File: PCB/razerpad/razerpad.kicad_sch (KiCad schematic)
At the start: 11 parts, among them SW1 SW_Push, SW2 SW_Push, SW3 SW_Push, SW4 RotaryEncoder_Switch, SW5 SW_Push, SW6 SW_Push, SW7 SW_Push, SW8 SW_Push, SW9 SW_Push, U1 XIAO-RP2040-DIP

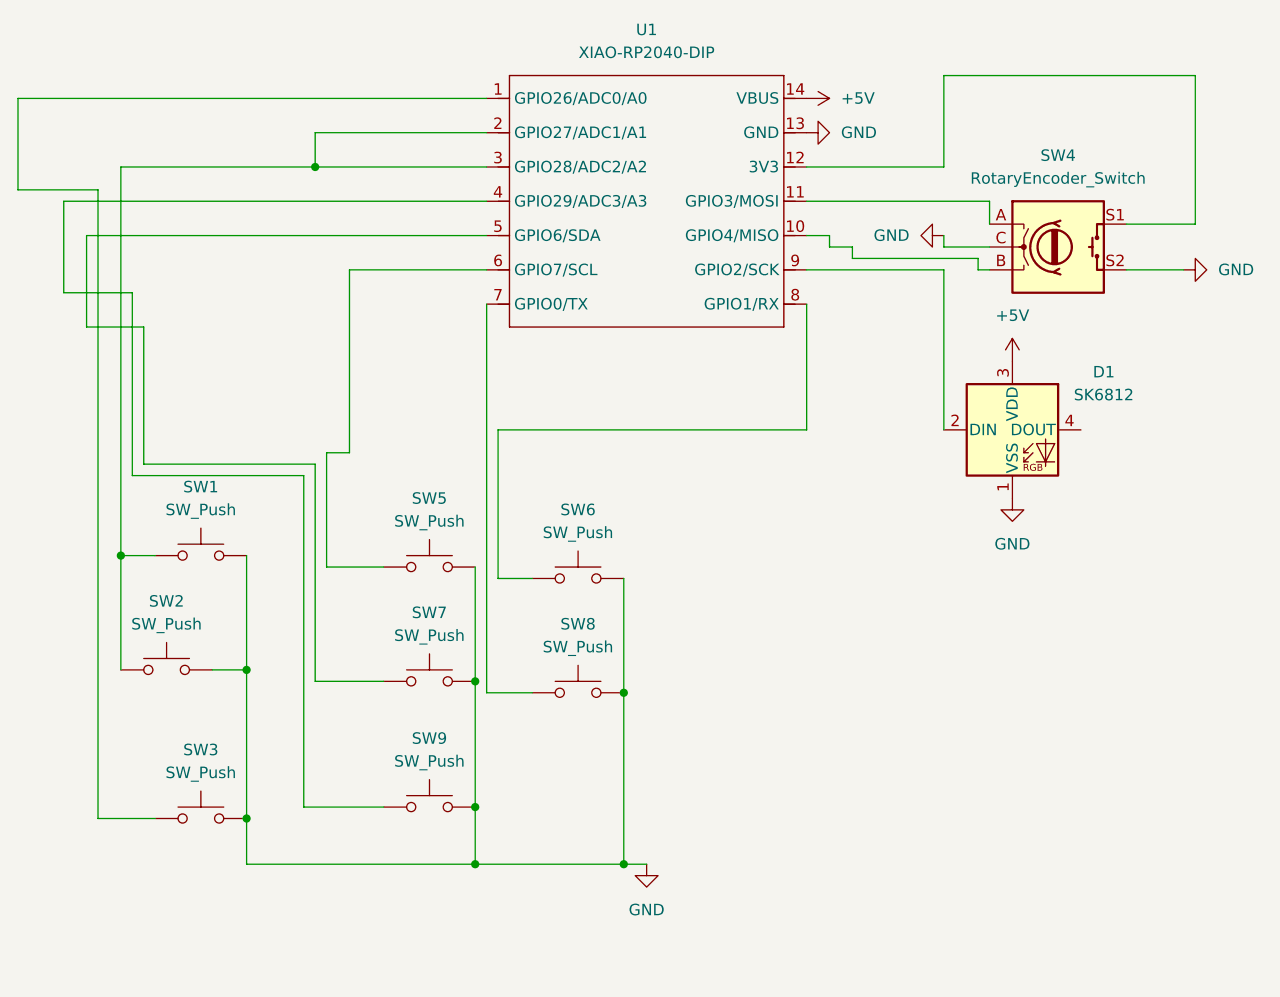
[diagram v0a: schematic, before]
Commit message: alright
Signed-off-by: Shubh <shubhisroking@proton.me>
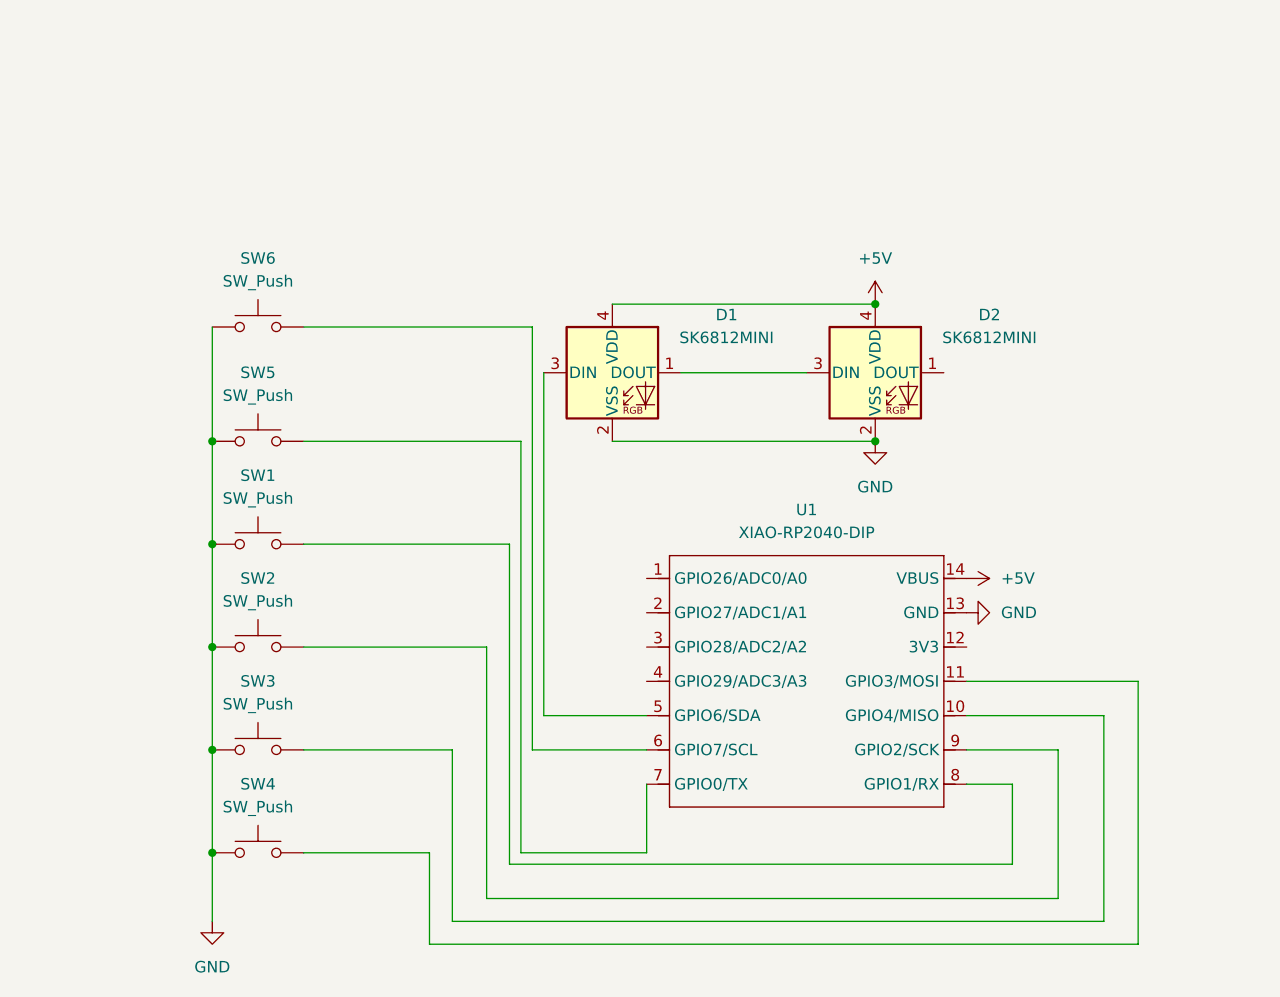
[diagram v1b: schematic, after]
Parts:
- removed D1: SK6812, LED_SMD:LED_SK6812_PLCC4_5.0x5.0mm_P3.2mm, symbol LED:SK6812
- removed SW4: RotaryEncoder_Switch, Rotary_Encoder:RotaryEncoder_Alps_EC11E-Switch_Vertical_H20mm, symbol Device:RotaryEncoder_Switch
- removed SW7, SW8, SW9: SW_Push, Button_Switch_Keyboard:SW_Cherry_MX_1.00u_PCB, symbol Switch:SW_Push
- added D1, D2: SK6812MINI, LED_SMD:LED_SK6812MINI_PLCC4_3.5x3.5mm_P1.75mm, symbol LED:SK6812MINI
- added SW4: SW_Push, Button_Switch_Keyboard:SW_Cherry_MX_1.00u_PCB, symbol Switch:SW_Push
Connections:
- net +5V: now also D1.4 (VDD), D2.4 (VDD)
- net GND: now also SW1.1, SW2.1, SW3.1, SW5.1, SW6.1, D1.2 (VSS), D2.2 (VSS), SW4.1; no longer SW1.2, SW2.2, SW3.2, SW5.2, SW6.2
- net at U1.5 (GPIO6/SDA): now also D1.3 (DIN)
- net at U1.7 (GPIO0/TX): now also SW5.2
- net at U1.11 (GPIO3/MOSI): now also SW4.2
- net at U1.10 (GPIO4/MISO): now also SW3.2
- net at U1.8 (GPIO1/RX): now also SW1.2; no longer SW6.1
- net at U1.1 (GPIO26/ADC0/A0): no longer SW3.1
- net at U1.6 (GPIO7/SCL): now also SW6.2; no longer SW5.1
- net at U1.9 (GPIO2/SCK): now also SW2.2
- new net: D1.1 (DOUT), D2.3 (DIN)
- now unconnected: U1.2 (GPIO27/ADC1/A1), U1.3 (GPIO28/ADC2/A2)
